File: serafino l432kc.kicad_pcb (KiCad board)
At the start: 4 copper layers, 17.8 x 35.6 mm, 33 parts, among them J1 USB_B_Micro, J2 Conn_01x14, J3 Conn_01x14, Q1 AO3401A, SW1 SW_Push, SW2 SW_Push, U1 AP2112K-3.3, U2 USBLC6-2SC6, U3 STM32L432KCUx, Y1 32.768K

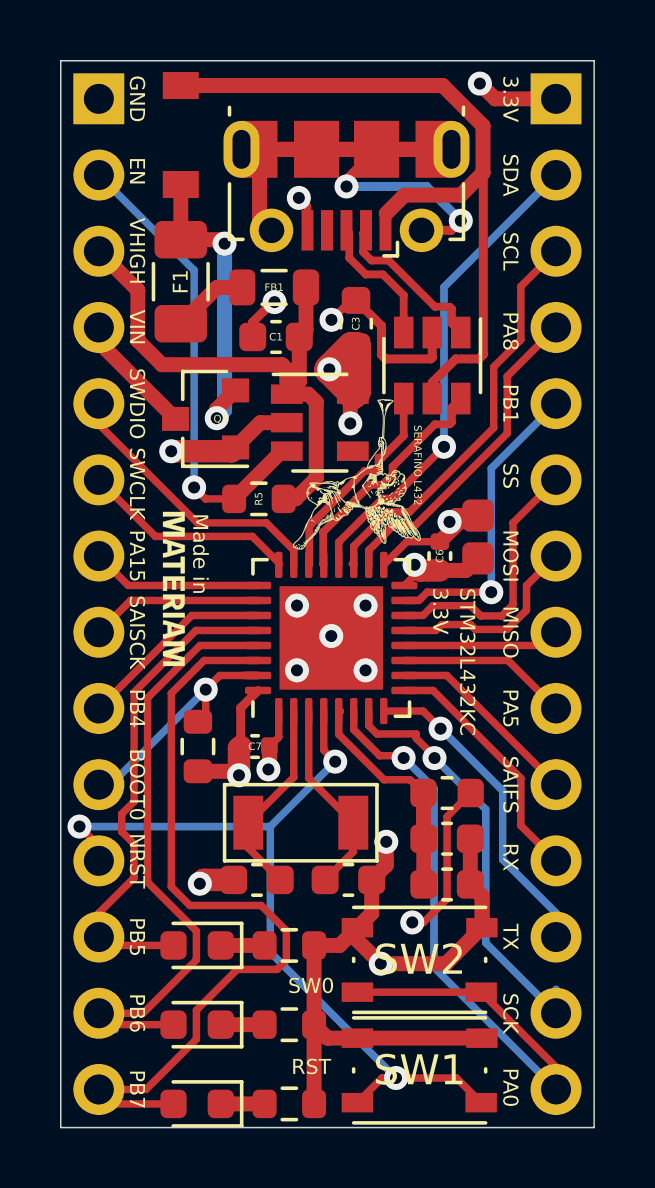
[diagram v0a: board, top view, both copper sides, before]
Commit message: version acorde con primer prototipo
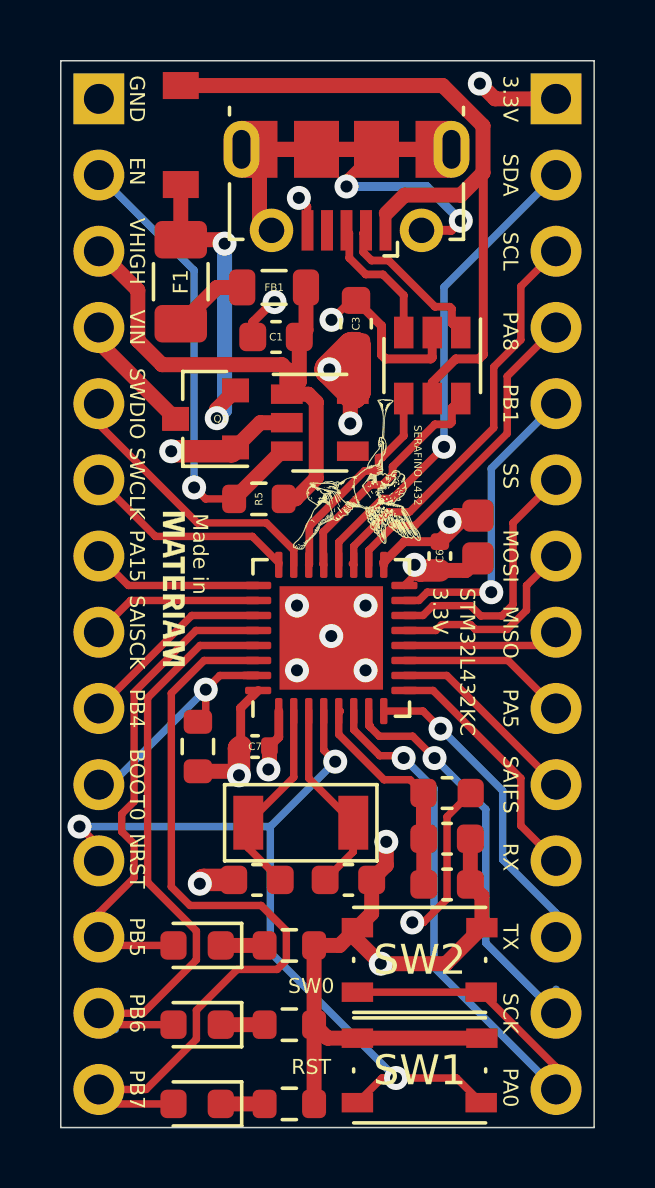
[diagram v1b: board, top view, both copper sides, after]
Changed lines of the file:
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@@
     (thickness 1.6)
     (drawings 41)
-    (tracks 374)
+    (tracks 377)
     (zones 0)
     (modules 33)
@@
   )
   (setup
-    (last_trace_width 0.25)
+    (last_trace_width 0.3)
     (user_trace_width 0.3)
     (user_trace_width 0.5)
@@
   (segment (start 200.6444 124.968) (end 201.4654 125.789) (width 0.25) (layer F.Cu) (net 3) (status 20))
   (segment (start 198.628 124.968) (end 200.6444 124.968) (width 0.25) (layer F.Cu) (net 3))
-  (segment (start 198.992 107.089) (end 200.0885 107.089) (width 0.25) (layer F.Cu) (net 4) (status 20))
-  (segment (start 198.219 107.862) (end 198.992 107.089) (width 0.25) (layer F.Cu) (net 4) (status 10))
   (segment (start 200.956 106.2215) (end 201.3585 106.2215) (width 0.5) (layer F.Cu) (net 4) (status 30))
   (segment (start 200.0885 107.089) (end 200.956 106.2215) (width 0.5) (layer F.Cu) (net 4) (status 30))
-  (segment (start 194.719 113.609) (end 194.409 113.919) (width 0.25) (layer F.Cu) (net 4) (status 20))
-  (segment (start 194.719 112.737) (end 194.719 113.609) (width 0.25) (layer F.Cu) (net 4) (status 10))
   (segment (start 197.188 100.7035) (end 197.2945 100.597) (width 0.5) (layer F.Cu) (net 4) (status 30))
   (segment (start 203.962 92.329) (end 203.454 92.329) (width 0.5) (layer F.Cu) (net 4) (status 30))
@@
   (segment (start 200.3298 118.994234) (end 199.541918 119.782116) (width 0.25) (layer F.Cu) (net 4))
   (segment (start 201.1173 115.4684) (end 200.3298 116.2559) (width 0.25) (layer F.Cu) (net 4) (status 10))
+  (segment (start 198.907304 107.089) (end 200.0885 107.089) (width 0.3) (layer F.Cu) (net 4))
+  (segment (start 198.219 107.777304) (end 198.907304 107.089) (width 0.3) (layer F.Cu) (net 4))
+  (segment (start 198.219 107.862) (end 198.219 107.777304) (width 0.3) (layer F.Cu) (net 4))
+  (segment (start 194.719 113.609) (end 194.409 113.919) (width 0.3) (layer F.Cu) (net 4))
+  (segment (start 194.719 112.737) (end 194.719 113.609) (width 0.3) (layer F.Cu) (net 4))
   (segment (start 195.219 114.943) (end 193.703 116.459) (width 0.25) (layer F.Cu) (net 5) (status 20))
   (segment (start 195.219 112.737) (end 195.219 114.943) (width 0.25) (layer F.Cu) (net 5) (status 10))
@@
   (segment (start 202.184 117.690002) (end 203.962 119.468002) (width 0.25) (layer B.Cu) (net 22) (status 20))
   (segment (start 202.184 115.395304) (end 202.184 117.690002) (width 0.25) (layer B.Cu) (net 22))
-  (segment (start 197.995988 113.49951) (end 199.30149 113.49951) (width 0.25) (layer F.Cu) (net 23))
-  (segment (start 197.719 113.222522) (end 197.995988 113.49951) (width 0.25) (layer F.Cu) (net 23))
   (segment (start 197.719 112.737) (end 197.719 113.222522) (width 0.25) (layer F.Cu) (net 23) (status 10))
   (via (at 199.911198 114.303214) (size 0.8) (drill 0.4) (layers F.Cu B.Cu) (net 23))
   (segment (start 199.883882 114.22888) (end 199.91578 114.22888) (width 0.25) (layer F.Cu) (net 23))
-  (segment (start 199.30149 113.646488) (end 199.883882 114.22888) (width 0.25) (layer F.Cu) (net 23))
-  (segment (start 199.30149 113.49951) (end 199.30149 113.646488) (width 0.25) (layer F.Cu) (net 23))
   (segment (start 203.962 122.008002) (end 203.962 122.809) (width 0.25) (layer B.Cu) (net 23) (status 30))
   (segment (start 201.618009 120.465009) (end 203.962 122.809) (width 0.25) (layer B.Cu) (net 23) (status 20))
   (segment (start 201.618009 116.010025) (end 201.618009 120.465009) (width 0.25) (layer B.Cu) (net 23))
   (segment (start 199.911198 114.303214) (end 201.618009 116.010025) (width 0.25) (layer B.Cu) (net 23))
+  (segment (start 199.182983 113.574999) (end 199.911198 114.303214) (width 0.25) (layer F.Cu) (net 23))
+  (segment (start 198.071477 113.574999) (end 199.182983 113.574999) (width 0.25) (layer F.Cu) (net 23))
+  (segment (start 197.76899 113.272512) (end 198.071477 113.574999) (width 0.25) (layer F.Cu) (net 23))
+  (segment (start 197.757478 113.222522) (end 197.76899 113.234034) (width 0.25) (layer F.Cu) (net 23))
+  (segment (start 197.76899 113.234034) (end 197.76899 113.272512) (width 0.25) (layer F.Cu) (net 23))
+  (segment (start 197.719 113.222522) (end 197.757478 113.222522) (width 0.25) (layer F.Cu) (net 23))
   (segment (start 197.219 113.358932) (end 198.084578 114.22451) (width 0.25) (layer F.Cu) (net 24))
   (segment (start 197.219 112.737) (end 197.219 113.358932) (width 0.25) (layer F.Cu) (net 24) (status 10))
